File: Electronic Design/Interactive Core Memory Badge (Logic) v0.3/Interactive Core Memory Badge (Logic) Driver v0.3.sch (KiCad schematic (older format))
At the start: 68 parts, among them J1 Conn_01x16_Female, J2 Conn_01x16_Female, Q10 MMBT4401LT1G, Q11 MMBT4403LT1G, Q12 MMBT4401LT1G, Q13 MMBT4403LT1G, Q14 MMBT4401LT1G, Q15 MMBT4403LT1G, Q16 MMBT4401LT1G, Q17 MMBT4403LT1G, Q18 MMBT4401LT1G, Q19 MMBT4403LT1G, Q2 MMBT4403LT1G, Q20 MMBT4401LT1G, Q21 MMBT4403LT1G, Q22 MMBT4401LT1G, Q3 MMBT4401LT1G, Q4 MMBT4401LT1G, Q5 MMBT4403LT1G, Q6 MMBT4401LT1G, Q7 MMBT4403LT1G, Q8 MMBT4401LT1G, Q9 MMBT4403LT1G

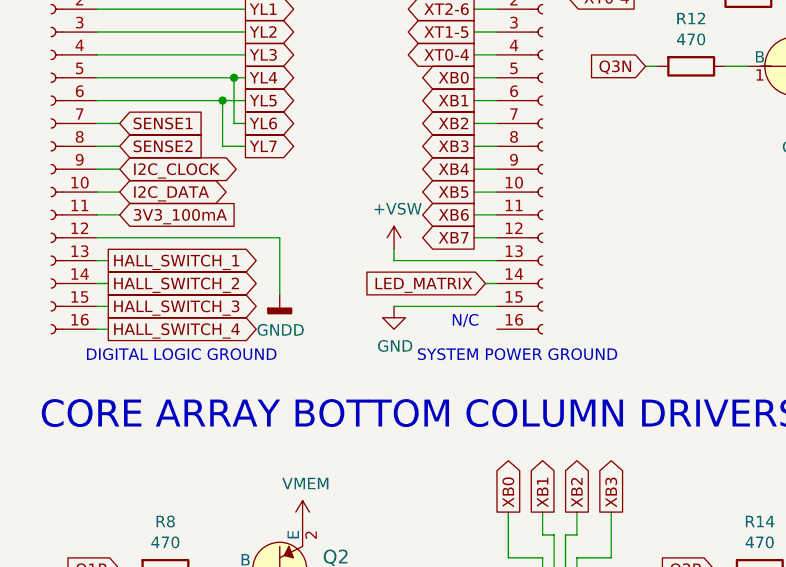
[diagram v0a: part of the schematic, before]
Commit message: Schematic refinement
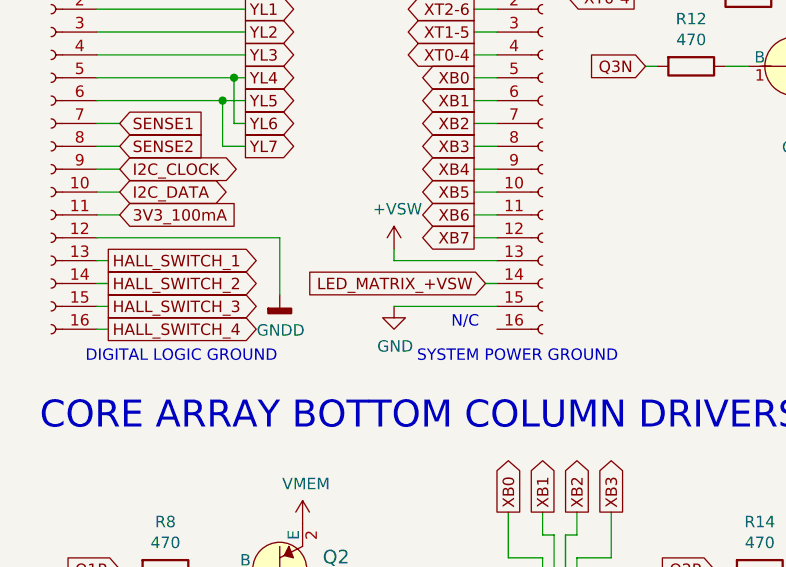
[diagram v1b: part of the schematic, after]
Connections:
- net LED_MATRIX renamed LED_MATRIX_+VSW
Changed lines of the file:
@@
 $Descr A 11000 8500
 encoding utf-8
-Sheet 4 6
+Sheet 2 5
 Title "Core 64 - Core Array Driver"
 Date "2020-03-15"
@@
 	900  2400 800  2400
 Text GLabel 2500 3000 0    50   Input ~ 0
-LED_MATRIX
+LED_MATRIX_+VSW
 Wire Wire Line
 	2500 3000 2550 3000
